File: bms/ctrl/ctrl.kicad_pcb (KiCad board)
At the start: 2 copper layers, 67 x 65 mm, 63 parts, among them J1 Conn_01x02_Female, J10 Conn_LEM_3, J11 Conn_01x02_Female, J12 Conn_01x04, J3 ScrewTerminal, J4 Conn_01x06, J5 Conn_01x04, J6 Conn_LEM_5, J7 Conn_01x02_Male, J8 Conn_01x02_Female, J9 Conn_01x03, Q5 DMN2058U-7, Q6 DMN2058U-7, U1 STH05_5V, U2 STH05_12, U3 VOS618A, U4 SN65HVD75DR, U5 Pico, U6 SN65HVD1050D

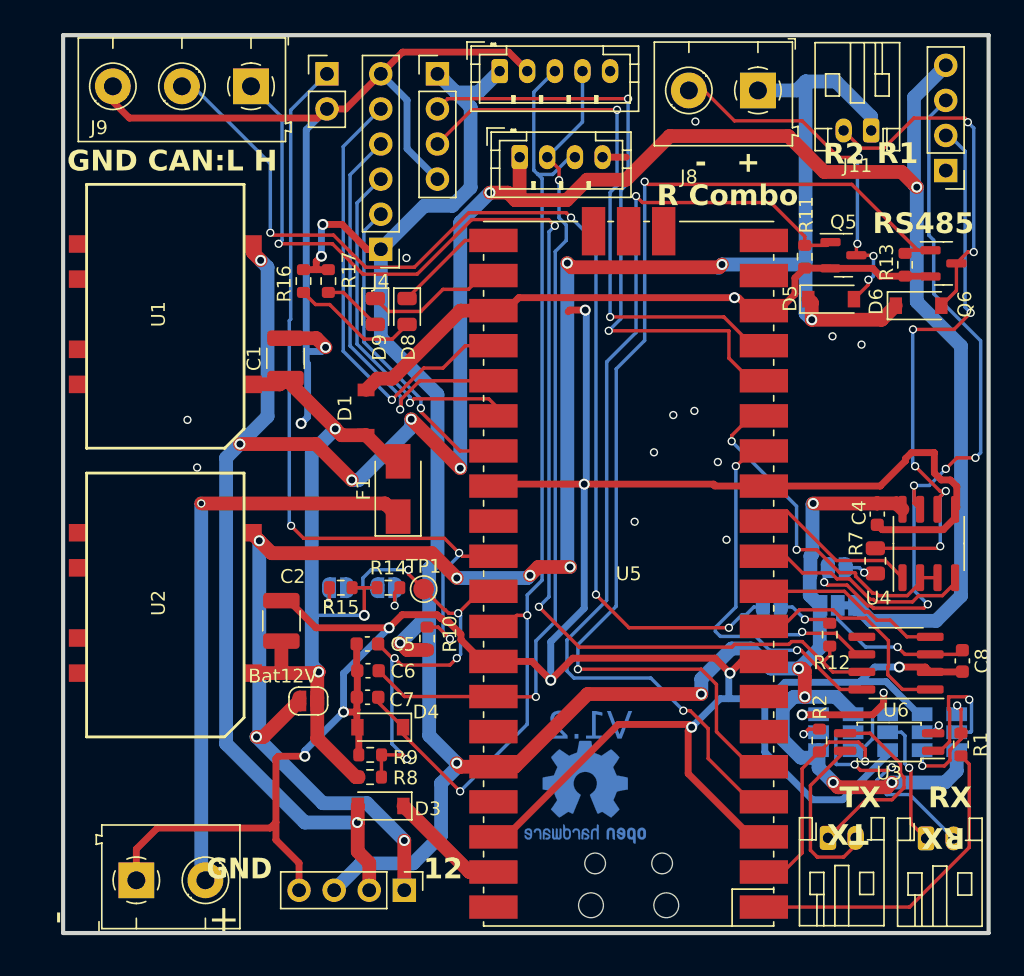
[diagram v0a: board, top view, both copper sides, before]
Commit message: Old check-in: ctrl
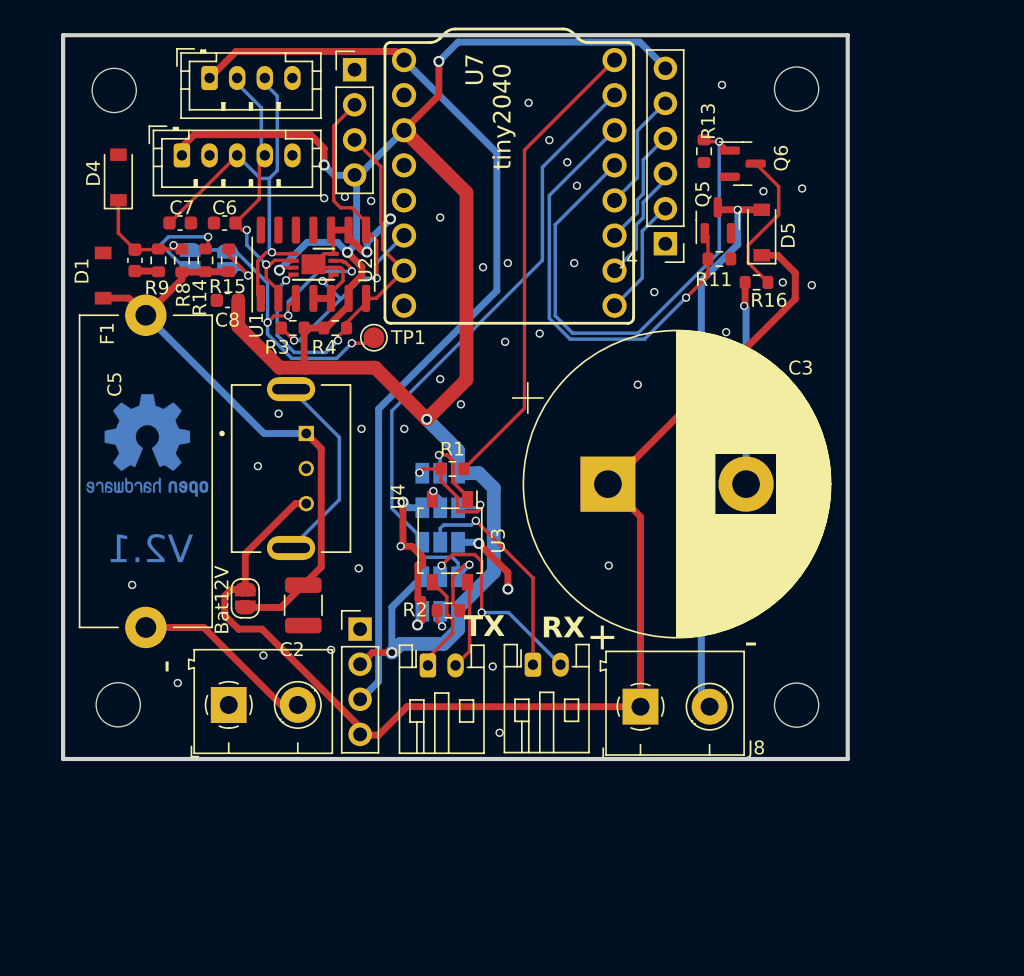
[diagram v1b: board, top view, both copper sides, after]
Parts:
- removed C1: CP_1µ_100V_0805, Resistor_SMD:R_1210_3225Metric
- removed C4: 100nF, Capacitor_SMD:C_0603_1608Metric
- removed D3: D_Schottky, Diode_SMD:D_SOD-123
- removed D6: 1N4148, Diode_SMD:D_SOD-123
- removed D8: LED_red, LED_SMD:LED_0805_2012Metric
- removed D9: LED_green, LED_SMD:LED_0805_2012Metric
- removed J11: Conn_01x02_Female, Connector_JST:JST_PH_S2B-PH-K_1x02_P2.00mm_Horizontal
- removed J3: ScrewTerminal, Connector_PinHeader_2.54mm:PinHeader_1x04_P2.54mm_Vertical
- removed J7: Conn_01x02_Male, Connector_PinHeader_2.54mm:PinHeader_1x02_P2.54mm_Vertical
- removed J9: Conn_01x03, localstuff:Conn_P5.0mm_3_Lumberg
- removed JP6: OptTermination, Jumper:SolderJumper-2_P1.3mm_Open_RoundedPad1.0x1.5mm
- removed JP7: CANBUS Volt Select, Jumper:SolderJumper-3_P1.3mm_Bridged12_RoundedPad1.0x1.5mm
- removed JP8: 24V, Jumper:SolderJumper-2_P1.3mm_Open_RoundedPad1.0x1.5mm
- removed R10: R_10k_0603, Resistor_SMD:R_0603_1608Metric
- removed R12: R_120_0603, Resistor_SMD:R_0603_1608Metric
- removed R17: R_510_0603, Resistor_SMD:R_0603_1608Metric
- removed R7: 120R, Resistor_SMD:R_0805_2012Metric
- removed U5: Pico, pico:RPi_Pico_SMD_TH
- removed U6: SN65HVD1050D, Package_SO:SOIC-8_3.9x4.9mm_P1.27mm
- added C3: CP_22m_16V, Capacitor_THT:CP_Radial_D22.0mm_P10.00mm_SnapIn, F.Cu at (84.4, 103.9)
- added R3: R_5k1_0603, Resistor_SMD:R_0603_1608Metric, F.Cu at (61.6, 92.6)
- added R4: R_5k1_0603, Resistor_SMD:R_0603_1608Metric, F.Cu at (64.7, 92.6)
- added REF**: MountingHole_3.2mm_M3, MountingHole:MountingHole_3.2mm_M3, F.Cu at (98.1, 75.3)
- added REF**: MountingHole_3.2mm_M3, MountingHole:MountingHole_3.2mm_M3, F.Cu at (98.1, 119.9)
- added REF**: MountingHole_3.2mm_M3, MountingHole:MountingHole_3.2mm_M3, F.Cu at (49.0, 119.9)
- added REF**: MountingHole_3.2mm_M3, MountingHole:MountingHole_3.2mm_M3, F.Cu at (48.7, 75.4)
- added U7: tiny2040, localstuff:tiny2040, F.Cu at (68.3, 80.8)
- C8: value CP_10µ_16V_0603 -> CP_100n_50V_0603
- F1: value Polyfuse 100V -> Fuse; footprint Diode_SMD:D_SMA -> Fuse:Fuseholder_Cylinder-5x20mm_Stelvio-Kontek_PTF78_Horizontal_Open
- R16: value R_560_0603 -> R_22_0603
- U1: value STH05_5V -> MCP3428; footprint localstuff:STH05 -> Package_SO:SOIC-14_3.9x8.7mm_P1.27mm
- U2: value STH05_12 -> MCP3426-xMC; footprint localstuff:STH05 -> Package_DFN_QFN:DFN-8-1EP_3x2mm_P0.5mm_EP1.75x1.45mm
- U3: footprint Package_SO:SOP-4_4.4x2.6mm_P1.27mm -> Package_SO:SO-4_4.4x4.3mm_P2.54mm
- U4: value SN65HVD75DR -> TSR_1-48150WI; footprint Package_SO:SOIC-8_3.9x4.9mm_P1.27mm -> localstuff:TSR_1-48150WI
- moved C8 59.3 mm to (56.9, 90.6), turned to 180 degrees
- moved U4 46.5 mm to (61.5, 102.8), turned to -90 degrees
- moved J8 45.4 mm to (86.8, 120.0), turned to 0 degrees
- moved D4 44.1 mm to (49.0, 81.7), turned to 90 degrees
- moved R1 41.9 mm to (73.2, 102.8), turned to 0 degrees
- moved JP1 41.8 mm to (72.3, 103.1), turned to 0 degrees
- moved REF** 40.4 mm to (51.1, 101.1) (x2)
- moved R8 39.8 mm to (53.6, 87.7), turned to 90 degrees
- moved R9 38.9 mm to (51.9, 87.7), turned to -90 degrees
- moved JP2 38.5 mm to (72.3, 105.6), turned to 0 degrees
- moved C7 36.9 mm to (53.5, 85.0), turned to 0 degrees
- moved JP4 35.2 mm to (72.3, 108.1), turned to 0 degrees
- moved U3 35.0 mm to (73.0, 108.0), turned to -90 degrees
- moved C6 34.0 mm to (56.7, 85.0)
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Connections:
- C8 pad 1: Net-(JP7-C) -> +3V3
- D4 pad 1: ADC_BAT_I -> ADC_BAT_U
- J12 pad 1: +12V -> GND
- J12 pad 2: +5V -> +3V3
- J12 pad 3: +3V3 -> +5V
- J12 pad 4: GND -> +12V
- J4 pad 1: +3V3 -> GND
- J4 pad 2: IO1 -> IO4
- J4 pad 3: IO2 -> IO3
- J4 pad 4: IO3 -> IO2
- J4 pad 5: IO4 -> IO1
- J4 pad 6: GND -> +3V3
- J5 pad 1: +3V3 -> GND
- J5 pad 2: I2C0_SDA -> I2C0_SCL
- J5 pad 3: I2C0_SCL -> I2C0_SDA
- J5 pad 4: GND -> +3V3
- Q6 pad 3: Net-(D6-A) -> Net-(Q6-D)
- R16 pad 1: +3V3 -> Net-(Q6-D)
- U1 pad 1: VBAT -> ADC_BAT_I
- U1 pad 10: unconnected-(U1-Enable) -> GND
- U1 pad 5: +5V -> GND
- U1 pad 6: unconnected-(U1-Trim) -> +3V3
- U1 pad 7: GND -> I2C0_SDA
- U2 pad 1: VBAT -> ADC_BAT_I
- U2 pad 5: +12V -> I2C0_SCL
- U2 pad 6: unconnected-(U2-Trim) -> GND
- U2 pad 7: GND -> ADC_BAT_U
- U4 pad 1: RS485_RX -> VBAT
- U4 pad 2: RS485_ENA -> GND
- U4 pad 3: RS485_ENA -> +12V
- U4 pad 4: RS485_TX -> Net-(U4-CASE_PIN)
- U4 pad 5: GND -> Net-(U4-CASE_PIN)
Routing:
- net GND: track 358.4 -> 37.4 mm, vias 26 -> 46
- net +5V: track 185.1 -> 68.4 mm, vias 8 -> 0
- net Net-(J9-Pin_1): track 90.3 -> 0.00 mm, vias 3 -> 0
- net Net-(J9-Pin_2): track 89.8 -> 0.00 mm, vias 5 -> 0
- net RESET: track 59.3 -> 0.00 mm, vias 3 -> 0
- net Net-(J3-Pin_3): track 53.8 -> 0.00 mm, vias 5 -> 0
- net +12V: track 136.6 -> 87.5 mm, vias 9 -> 0
- net Net-(J3-Pin_2): track 41.9 -> 0.00 mm, vias 5 -> 0
- net RELAY2: track 78.6 -> 37.7 mm, vias 2 -> 1
- net ADC_BAT_I: track 69.8 -> 28.9 mm, vias 2 -> 1
- net ADC_REF_I: track 60.0 -> 21.3 mm
- net RELAY1: track 71.0 -> 32.8 mm, vias 2 -> 1
- net Net-(J1-Pin_2): track 42.0 -> 13.3 mm, vias 1 -> 0
- net RX_BAT: track 22.6 -> 50.2 mm
- net CAN_S: track 26.5 -> 0.00 mm, vias 2 -> 0
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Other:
- board size 67 x 65 mm -> 56.8 x 52.4 mm
- board text added: "- + Relais"
- board text added: "V2.1"
- board text removed: "- + R Combo"
- board text removed: "5v CAN 3.3v"
- board text removed: "CAN"
- board text removed: "GND CAN:L H"
- board text removed: "R1"
- board text removed: "R2"
- board text removed: "RS485"
- board text removed: "RS485 term"
- board text removed: "V1.2"
- board text removed: "open: 48V"
